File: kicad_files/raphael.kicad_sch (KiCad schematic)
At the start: 345 parts

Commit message: Organize schematic, preparing for release
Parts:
- C1: value (none) -> 10u; footprint (none) -> Capacitor_SMD:C_0402_1005Metric
- C10: value (none) -> 10u; footprint (none) -> acheron_Components:CP_EIA-3216-10_Kemet-I_Pad1.58x1.35mm_HandSolder
- C11, C16: value (none) -> 4.7u; footprint (none) -> Capacitor_SMD:C_0402_1005Metric
- C12: value (none) -> 10n; footprint (none) -> Capacitor_SMD:C_0402_1005Metric
- C13, C14: value (none) -> 16p; footprint (none) -> Capacitor_SMD:C_0402_1005Metric
- C15, C2, C6, C7, C8, C9: value (none) -> 100n; footprint (none) -> Capacitor_SMD:C_0402_1005Metric
- C3, C4: value (none) -> 1u; footprint (none) -> Capacitor_SMD:C_0805_2012Metric
- C5: value (none) -> 10n; footprint (none) -> Capacitor_SMD:C_0805_2012Metric
- D1, D10, D11, D12, D13, D14, D15, D16, D17, D18, D19, D20, D21, D22, D23, D24, D25, D26, D27, D28, D29, D3, D30, D31, D32, D33, D34, D35, D36, D37, D38, D39, D4, D40, D41, D42, D43, D44, D45, D46, D47, D48, D49, D5, D50, D51, D52, D53, D54, D55, D56, D57, D58, D59, D6, D60, D61, D62, D63, D64, D65, D66, D67, D68, D7, D8, D9: value (none) -> 1N4148W; footprint (none) -> acheron_Components:D_SOD-123
- D2: value (none) -> B5819W-SL; footprint (none) -> acheron_Components:D_SOD-123
- F1: value (none) -> nSMD100-16V; footprint (none) -> Fuse:Fuse_1206_3216Metric
- FB1: value (none) -> GZ2012D601TF; footprint (none) -> Inductor_SMD:L_0805_2012Metric
- GR1: value (none) -> Raphael huge logo; footprint (none) -> raphael_library:raphael_logo_56.9x84mm
- GR2: value (none) -> Raphael plated logo; footprint (none) -> raphael_library:raphael_plated_logo_12x17.7mm
- GR3: value (none) -> Rapahel letters; footprint (none) -> raphael_library:raphael_logo_letters_41x2.5mm
- GR4: value (none) -> Rapahel label; footprint (none) -> raphael_library:raphael_label_191x3mm
- J1: value (none) -> A1001WR-S-04P; footprint (none) -> acheron_Connectors:SM04B-SRSS-TB(LF)(SN)_mounting-reliefs
- J2: value (none) -> TYPE-C-31-M-12; footprint (none) -> acheron_Connectors:TYPE-C-31-M-12
- LED1, LED10, LED11, LED12, LED13, LED14, LED15, LED16, LED17, LED18, LED19, LED2, LED20, LED21, LED22, LED23, LED24, LED25, LED26, LED27, LED28, LED29, LED3, LED30, LED31, LED32, LED33, LED34, LED35, LED36, LED37, LED38, LED39, LED4, LED40, LED41, LED42, LED43, LED44, LED45, LED46, LED47, LED48, LED49, LED5, LED50, LED51, LED52, LED53, LED54, LED55, LED56, LED57, LED58, LED59, LED6, LED60, LED61, LED62, LED63, LED64, LED65, LED66, LED67, LED68, LED69, LED7, LED70, LED71, LED72, LED73, LED74, LED75, LED76, LED77, LED8, LED9: value (none) -> LED; footprint (none) -> acheron_Components:LED_THT_2.54mm
- Q1: value (none) -> AO3401A; footprint (none) -> Package_TO_SOT_SMD:SOT-23
- Q2, Q3: value (none) -> 2N7002; footprint (none) -> Package_TO_SOT_SMD:SOT-23
- R1: value (none) -> 330k; footprint (none) -> Resistor_SMD:R_0402_1005Metric
- R10, R16, R19, R3, R9: value (none) -> 10k; footprint (none) -> Resistor_SMD:R_0402_1005Metric
- R11, R12: value (none) -> 4.7k; footprint (none) -> Resistor_SMD:R_0402_1005Metric
- R13: value (none) -> 1.5k; footprint (none) -> Resistor_SMD:R_0402_1005Metric
- R14, R15: value (none) -> 5.1k; footprint (none) -> Resistor_SMD:R_0402_1005Metric
- R17, R18: value (none) -> 100; footprint (none) -> Resistor_SMD:R_0402_1005Metric
- R2: value (none) -> 1M; footprint (none) -> Resistor_SMD:R_0402_1005Metric
- R20, R21, R22, R23, R24, R25, R26, R27, R28, R29, R30, R31, R32, R33, R34, R35, R36, R37, R38, R39, R40, R41, R42, R43, R44, R45, R46, R47, R48, R49, R50, R51, R52, R53, R54, R55, R56, R57, R58, R59, R60, R61, R62, R63, R64, R65, R66, R67, R68, R69, R70, R71, R72, R73, R74, R77, R78, R79, R80, R81, R82, R83, R84, R85, R86, R87: value (none) -> 1k; footprint (none) -> Resistor_SMD:R_0805_2012Metric
- R4, R5, R6: value (none) -> 100R; footprint (none) -> Resistor_SMD:R_0402_1005Metric
- R7, R8: value (none) -> 100k; footprint (none) -> Resistor_SMD:R_0805_2012Metric
- R75: value (none) -> 100R; footprint (none) -> Resistor_SMD:R_0805_2012Metric
- R76: value (none) -> 10k; footprint (none) -> Resistor_SMD:R_0805_2012Metric
- SW1: value (none) -> K2-1187SQ-A4SW-06; footprint (none) -> acheron_Hardware:K2-1187SQ-A4SW-06
- SW10, SW11, SW12, SW13, SW14, SW15, SW17, SW18, SW19, SW2, SW20, SW21, SW22, SW23, SW24, SW25, SW26, SW27, SW29, SW3, SW30, SW31, SW32, SW33, SW34, SW35, SW36, SW37, SW38, SW39, SW4, SW40, SW44, SW45, SW46, SW47, SW48, SW49, SW5, SW50, SW51, SW52, SW53, SW54, SW56, SW6, SW68, SW7, SW72, SW74, SW78, SW8, SW9: value (none) -> Mechanical_Switch; footprint (none) -> acheron_MX_soldermask:MX100
- SW16: value (none) -> Mechanical_Switch; footprint (none) -> acheron_MX_soldermask:MX200
- SW28, SW67, SW69, SW71, SW73, SW75: value (none) -> Mechanical_Switch; footprint (none) -> acheron_MX_soldermask:MX150
- SW41: value (none) -> Mechanical_Switch; footprint (none) -> acheron_MX_soldermask:MX225R
- SW42: value (none) -> Mechanical_Switch; footprint (none) -> acheron_MX_soldermask:MX_ISOEnter_Horizontal
- SW43: value (none) -> Mechanical_Switch; footprint (none) -> acheron_MX_soldermask:MX225
- SW55: value (none) -> Mechanical_Switch; footprint (none) -> acheron_MX_soldermask:MX275
- SW57, SW59, SW60, SW61, SW63, SW64, SW65, SW66, SW77: value (none) -> Mechanical_Switch; footprint (none) -> acheron_MX_soldermask:MX125
- SW58, SW76: value (none) -> Mechanical_Switch; footprint (none) -> acheron_MX_soldermask:MX175
- SW62: value (none) -> Mechanical_Switch; footprint (none) -> acheron_MX_soldermask:MX625R
- SW70: value (none) -> Mechanical_Switch; footprint (none) -> acheron_MX_soldermask:MX700R
- U1: value (none) -> USBLC6-2SC6; footprint (none) -> acheron_Components:SOT-23-6
- U2: value (none) -> 2N7002DW; footprint (none) -> acheron_Components:SOT-363_SC-70-6
- U3: value (none) -> SGM2007-3.3XN5/TR; footprint (none) -> acheron_Components:SOT-23-5
- U4: value (none) -> BL24C256A-SFRC; footprint (none) -> acheron_Components:TSSOP-8_4.4x3mm_P0.65mm
- U5: value (none) -> STM32F411CEU6; footprint (none) -> acheron_Components:STM_UFQFPN-48_LQFP-48-1EP_7x7mm_P0.5mm_HandSoldering_ThermalReliefs
- X1: value (none) -> ARM JTAG; footprint (none) -> acheron_Connectors:PinHeader_2x5_P2.54mm_Vertical_Staggered
- X2: footprint (none) -> acheron_Connectors:PinHeader_1x3_staggered_P2.54mm_Vertical
- Y1: value (none) -> 7325-0800A2010-00; footprint (none) -> acheron_Components:Crystal_SMD_3225-4Pin_3.2x2.5mm
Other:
- note added: "GRAPHICS"
- note added: "USB"
- moved on the sheet: C1, C10, C11, C12, C13, C14, C15, C16, C2, C3, C4, C5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

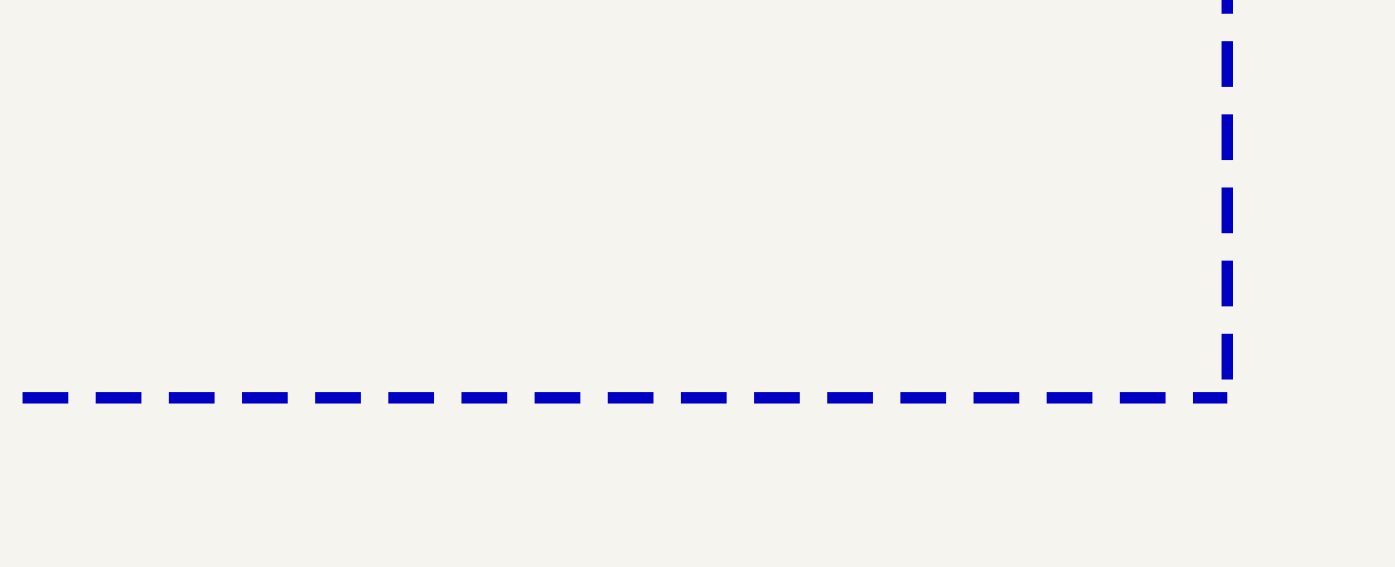
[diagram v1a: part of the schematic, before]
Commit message: Edit metadata, release
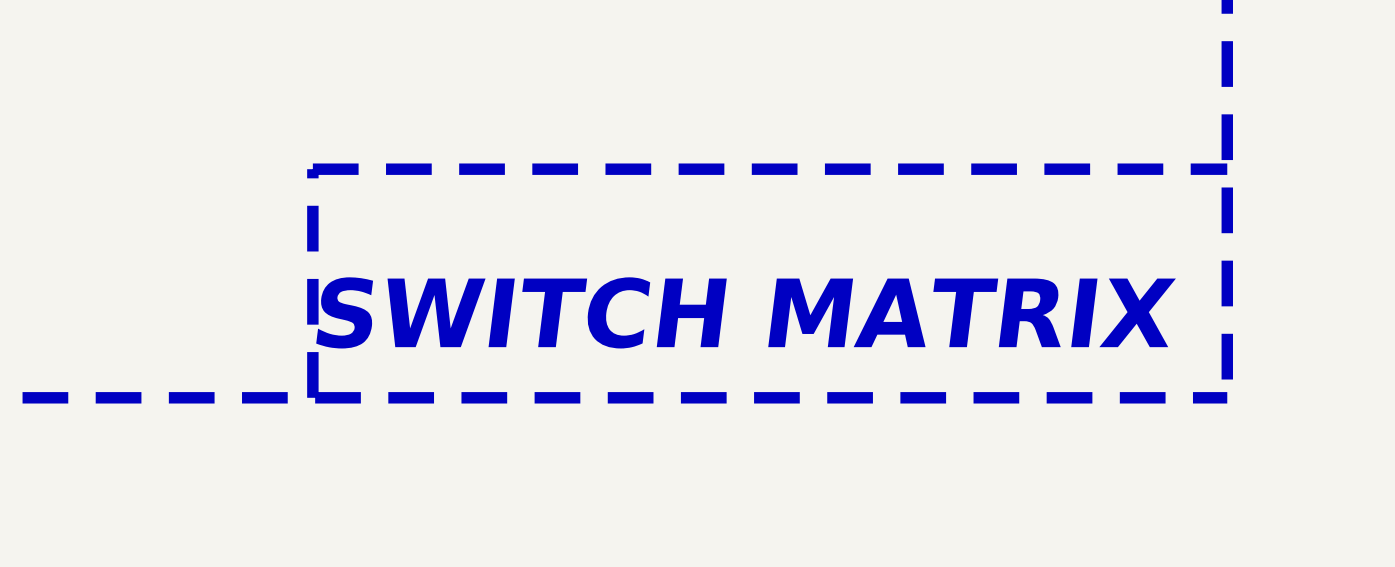
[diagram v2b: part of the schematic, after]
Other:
- note added: "SWITCH MATRIX"
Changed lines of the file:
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@@
     (stroke (width 0) (type solid) (color 0 0 0 0))
+  )
+  (polyline (pts (xy 412.75 762) (xy 412.75 736.6))
+    (stroke (width 1.27) (type dash) (color 0 0 0 0))
   )
   (polyline (pts (xy 533.4 552.45) (xy 635 552.45))
@@
   (wire (pts (xy 165.735 573.405) (xy 167.005 573.405))
     (stroke (width 0) (type default) (color 0 0 0 0))
+  )
+  (polyline (pts (xy 412.75 736.6) (xy 514.35 736.6))
+    (stroke (width 1.27) (type dash) (color 0 0 0 0))
   )
   (wire (pts (xy 142.24 107.95) (xy 142.24 109.22))
@@
     (effects (font (size 7.62 7.62) (thickness 1.524) bold italic) (justify right bottom))
   )
+  (text "SWITCH MATRIX" (at 508 757.555 180)
+    (effects (font (size 7.62 7.62) (thickness 1.524) bold italic) (justify right bottom))
+  )
